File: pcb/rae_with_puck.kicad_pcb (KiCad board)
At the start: 2 copper layers, 126.9 x 99.3 mm, 40 parts

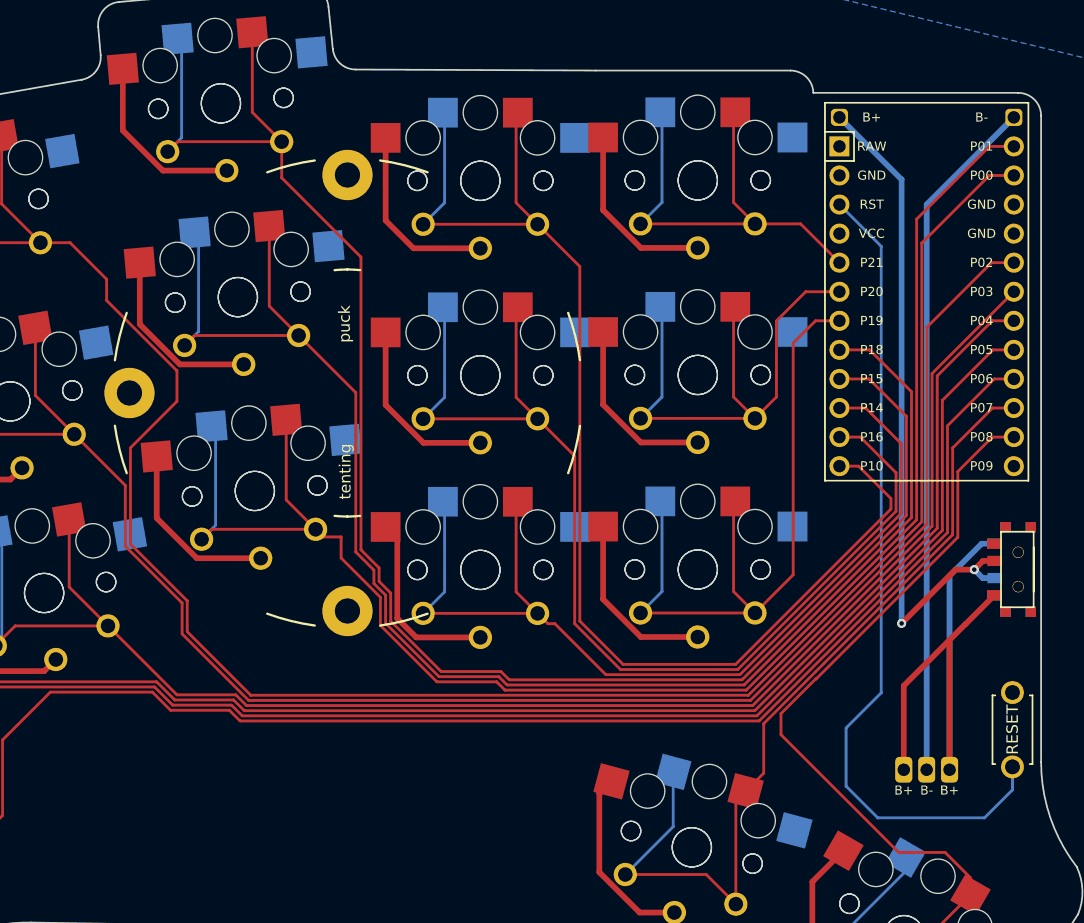
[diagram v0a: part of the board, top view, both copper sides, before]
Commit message: add gerber files
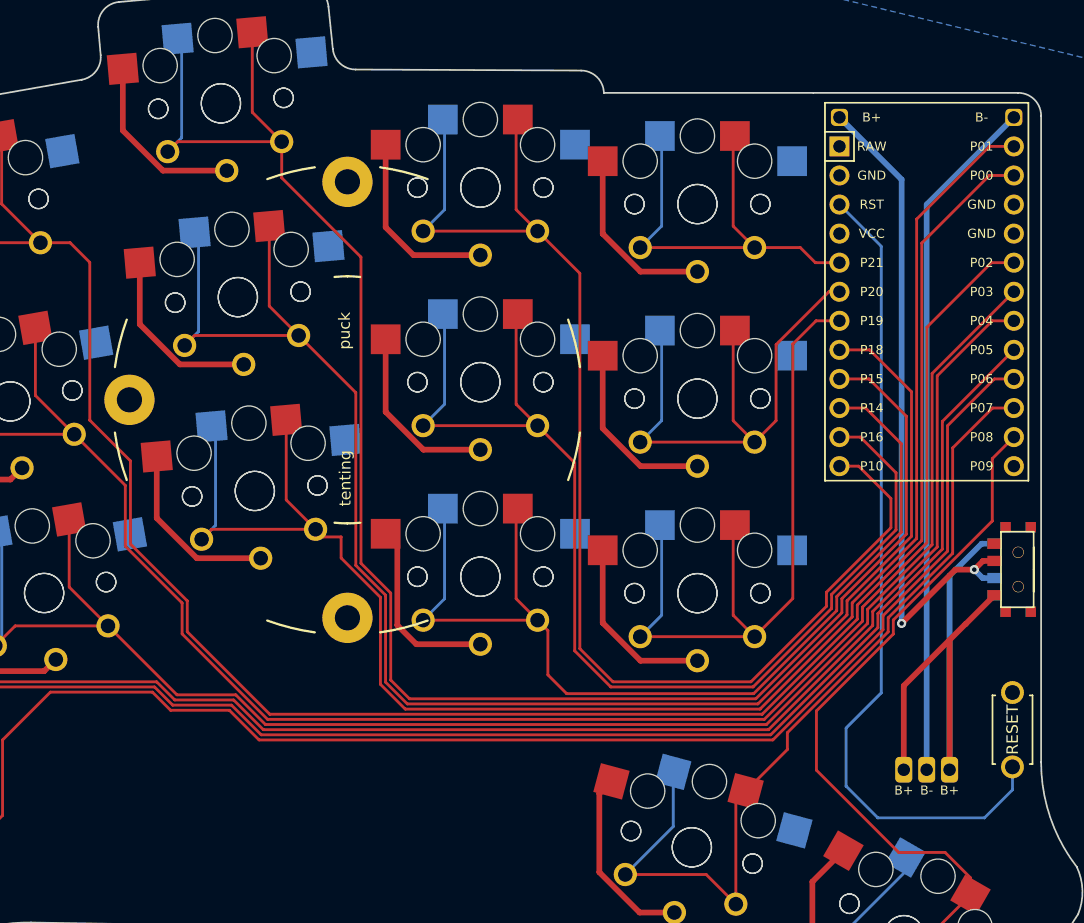
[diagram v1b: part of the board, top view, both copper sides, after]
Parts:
- moved S25 2.07 mm to (134.4, -71.2)
- moved S26 2.07 mm to (134.4, -71.2)
- moved S27 2.07 mm to (134.4, -88.2)
- moved S28 2.07 mm to (134.4, -88.2)
- moved S29 2.07 mm to (134.4, -105.2)
- moved S30 2.07 mm to (134.4, -105.2)
- moved REF** 0.60 mm to (103.8, -88.1)
- moved S19 0.60 mm to (115.4, -72.7)
- moved S20 0.60 mm to (115.4, -72.7)
- moved S21 0.60 mm to (115.4, -89.7)
- moved S22 0.60 mm to (115.4, -89.7)
- moved S23 0.60 mm to (115.4, -106.7)
- moved S24 0.60 mm to (115.4, -106.7)
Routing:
- net P1: track 135.9 -> 141.9 mm
- net P18: track 132.8 -> 138.9 mm
- net P15: track 146.3 -> 152.4 mm
- net P14: track 84.3 -> 89.4 mm
- net P10: track 108.9 -> 112.6 mm
- net P16: track 96.0 -> 99.8 mm
- net P8: track 90.5 -> 86.8 mm
- net P4: track 169.1 -> 172.2 mm
- net P6: track 154.1 -> 157.1 mm
- net P3: track 136.5 -> 139.5 mm
- net P2: track 154.0 -> 157.0 mm
- net P19: track 61.0 -> 63.0 mm
- net P5: track 150.9 -> 152.9 mm
- net P20: track 47.0 -> 47.9 mm
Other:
- outline, holes or cut-outs redrawn
